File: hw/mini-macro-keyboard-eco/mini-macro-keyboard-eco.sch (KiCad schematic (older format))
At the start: 32 parts, among them J0 USB, J1 DEBUG_SWD, SW1 SW_Cherry_MX_1.00u_PCB, SW2 SW_Cherry_MX_1.00u_PCB, SW3 SW_Cherry_MX_1.00u_PCB, SW5 LAYOUT, SW6 BACKLIGHT, U1 USBLC6-2SC6, U2 XC6206P322MR, U3 STM32F070F6P6, Y1 16 MHz

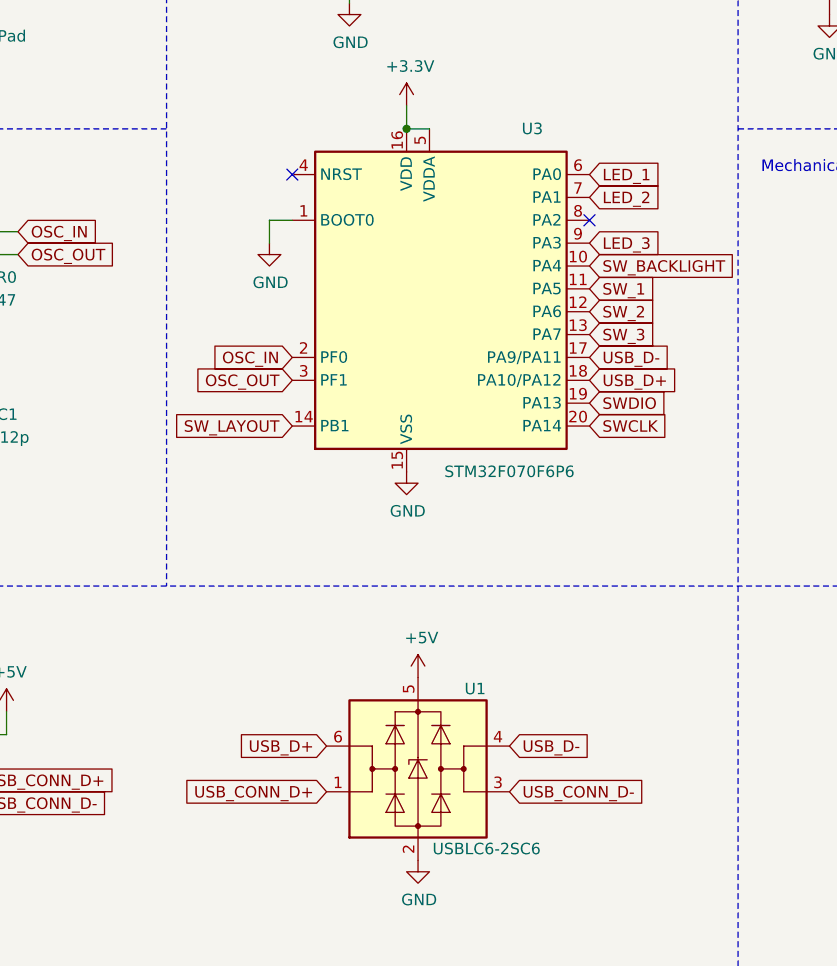
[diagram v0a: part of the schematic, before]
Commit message: feat(hw): add rooting
Signed-off-by: Ivan Kovalenko <s1ckretbox@gmail.com>
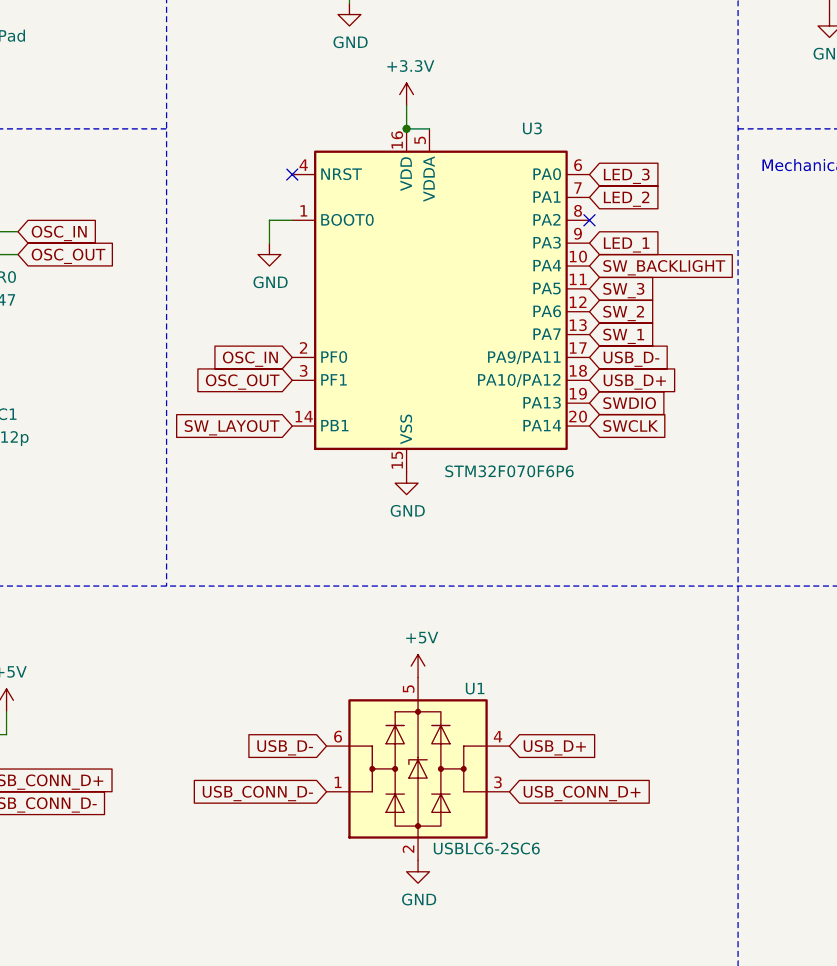
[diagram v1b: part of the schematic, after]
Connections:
- net LED_1: now also U3.9 (PA3); no longer U3.6 (PA0)
- net LED_3: now also U3.6 (PA0); no longer U3.9 (PA3)
- net SW_1: now also U3.13 (PA7); no longer U3.11 (PA5)
- net SW_3: now also U3.11 (PA5); no longer U3.13 (PA7)
- net USB_CONN_D+: now also U1.3 (I/O2); no longer U1.1 (I/O1)
- net USB_CONN_D-: now also U1.1 (I/O1); no longer U1.3 (I/O2)
- net USB_D+: now also U1.4 (I/O2); no longer U1.6 (I/O1)
- net USB_D-: now also U1.6 (I/O1); no longer U1.4 (I/O2)
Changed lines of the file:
@@
 Text GLabel 4350 3000 2    50   Input ~ 0
 USB_D-
-Text GLabel 4350 2500 2    50   Input ~ 0
+Text GLabel 4350 2200 2    50   Input ~ 0
 LED_3
 Text GLabel 4350 2300 2    50   Input ~ 0
 LED_2
-Text GLabel 4350 2200 2    50   Input ~ 0
+Text GLabel 4350 2500 2    50   Input ~ 0
 LED_1
-Text GLabel 4350 2700 2    50   Input ~ 0
+Text GLabel 4350 2900 2    50   Input ~ 0
 SW_1
 Text GLabel 4350 2800 2    50   Input ~ 0
 SW_2
-Text GLabel 4350 2900 2    50   Input ~ 0
+Text GLabel 4350 2700 2    50   Input ~ 0
 SW_3
 Text GLabel 3050 3100 0    50   Input ~ 0
@@
 Text GLabel 1650 4950 2    50   Input ~ 0
 USB_CONN_D-
-Text GLabel 3200 4900 0    50   Input ~ 0
+Text GLabel 4000 4900 2    50   Input ~ 0
 USB_CONN_D+
 $Comp
@@
 	1    0    0    -1
 $EndComp
+Text GLabel 4000 4700 2    50   Input ~ 0
+USB_D+
+Text GLabel 3200 4900 0    50   Input ~ 0
+USB_CONN_D-
 Text GLabel 3200 4700 0    50   Input ~ 0
-USB_D+
-Text GLabel 4000 4900 2    50   Input ~ 0
-USB_CONN_D-
-Text GLabel 4000 4700 2    50   Input ~ 0
 USB_D-
 Text GLabel 7650 900  0    50   Input ~ 0
